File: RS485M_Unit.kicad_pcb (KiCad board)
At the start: 2 copper layers, 20.6 x 28 mm, 30 parts, among them CN1 CON_GROVE, J1 Conn_01x04, SW1 SW_Push, U1 WB485E, U2 TD1466A, U4 MCU_STC8G1Kxx-8P

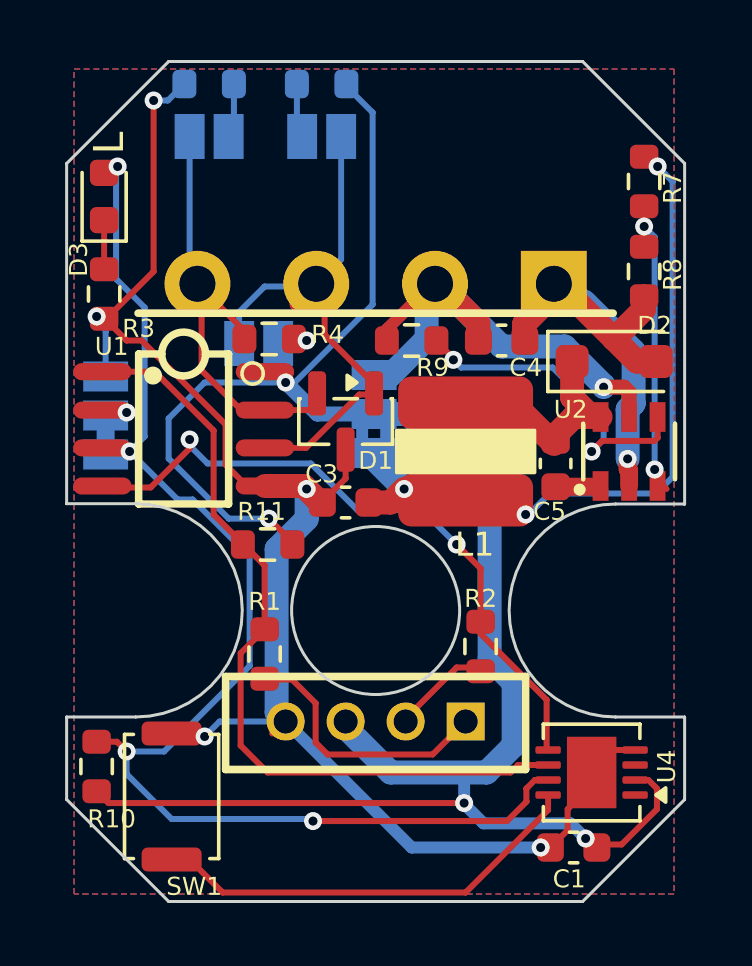
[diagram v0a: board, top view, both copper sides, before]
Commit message: update readme
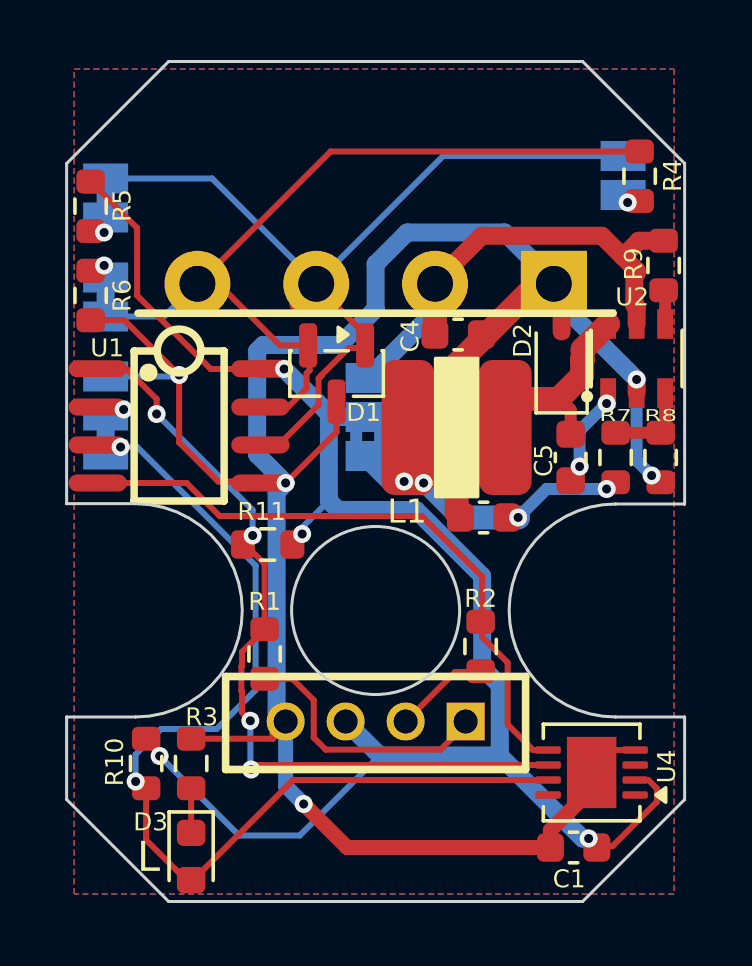
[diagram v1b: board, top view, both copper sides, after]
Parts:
- removed SW1: SW_Push, Button_Switch_SMD:SW_Push_SPST_NO_Alps_SKRK
- D2: footprint Diode_SMD:D_SOD-123F -> Diode_SMD:D_SOD-323F
- JP6, JP7: value Jumper_2_Open -> Jumper_2_Bridged; footprint Jumper:SolderJumper-2_P1.3mm_Open_Pad1.0x1.5mm -> Jumper:SolderJumper-2_P1.3mm_Bridged_Pad1.0x1.5mm
- R5, R6: moved to F.Cu
- moved D3 22.2 mm to (4.15, 26.5), turned to -90 degrees
- moved R3 15.9 mm to (4.15, 23.4), turned to 90 degrees
- moved R4 13.5 mm to (19.1, 3.83), turned to 90 degrees
- moved JP5 13.4 mm to (18.6, 3.80), turned to 90 degrees
- moved R7 9.25 mm to (18.3, 13.2), turned to -90 degrees
- moved R9 8.76 mm to (19.9, 6.80), turned to -90 degrees
- moved R5 8.71 mm to (0.80, 4.83), turned to -90 degrees
- moved R6 8.08 mm to (0.80, 7.80), turned to 90 degrees
- moved JP6 7.49 mm to (1.30, 4.55), turned to -90 degrees
- moved JP7 6.37 mm to (1.30, 7.85), turned to 90 degrees
- moved R8 6.22 mm to (19.8, 13.2)
- moved C3 4.63 mm to (13.9, 15.2)
- moved U2 3.11 mm to (19.0, 9.90)
- moved D2 1.75 mm to (16.5, 10.1), turned to 90 degrees
- moved R10 1.65 mm to (2.65, 23.4), turned to -90 degrees
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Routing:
- net +5V: track 70.1 -> 55.4 mm
- net /SW: track 14.7 -> 0.00 mm
- net GND: track 66.0 -> 79.9 mm, vias 6 -> 5
- net /BUS_B: track 15.0 -> 28.1 mm
- net Net-(JP9-A): track 21.7 -> 9.44 mm, vias 3 -> 4
- net /BUS_A: track 20.3 -> 31.1 mm
- net Net-(U2-EN): track 10.9 -> 1.07 mm, vias 2 -> 0
- net /TX_EN: track 42.8 -> 33.9 mm, vias 4 -> 2
- net Net-(U2-FB): track 10.0 -> 2.90 mm, vias 2 -> 0
- net Net-(U2-BST): track 1.48 -> 3.07 mm, vias 0 -> 2
- net Net-(JP6-B): track 1.78 -> 0.47 mm, vias 0 -> 1
- net Net-(JP7-B): track 1.78 -> 0.52 mm, vias 0 -> 1
- net Net-(JP5-A): track 1.49 -> 0.31 mm
- net /RXD: track 22.1 -> 21.0 mm, vias 2 -> 0
- net Net-(D2-K): track 5.35 -> 6.23 mm
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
